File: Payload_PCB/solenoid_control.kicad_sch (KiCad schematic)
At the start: 9 parts, among them Q2 NMOS, Q29 NMOS

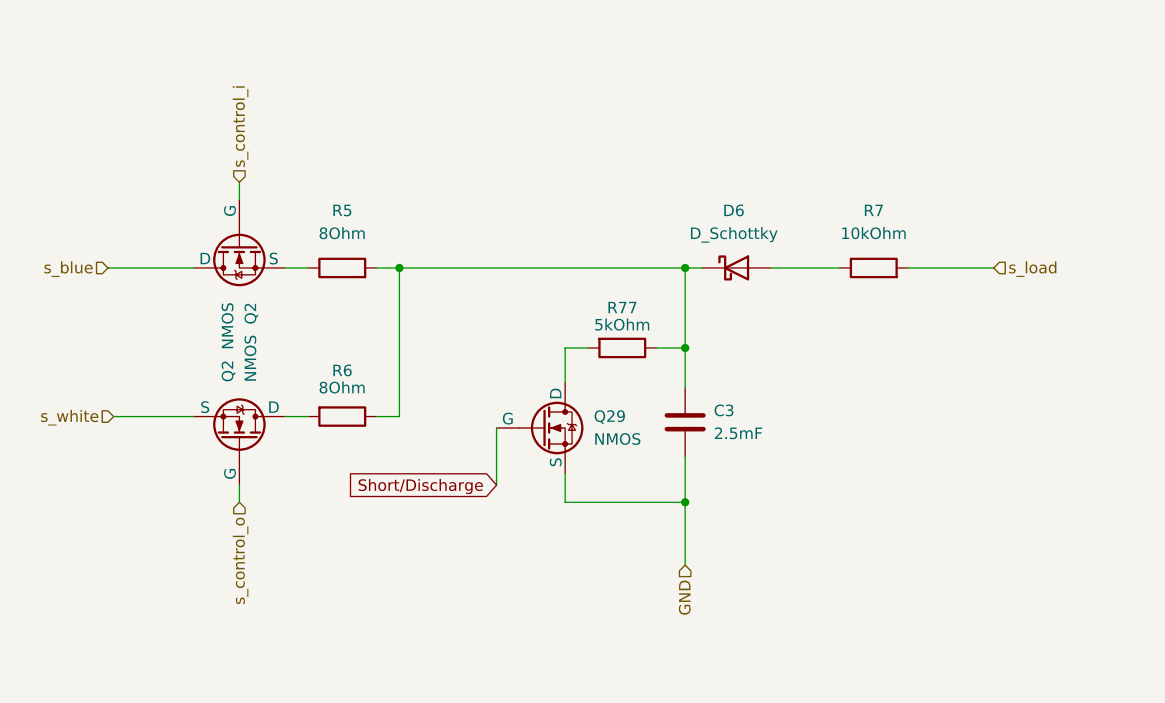
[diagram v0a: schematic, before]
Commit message: Added some actual parts
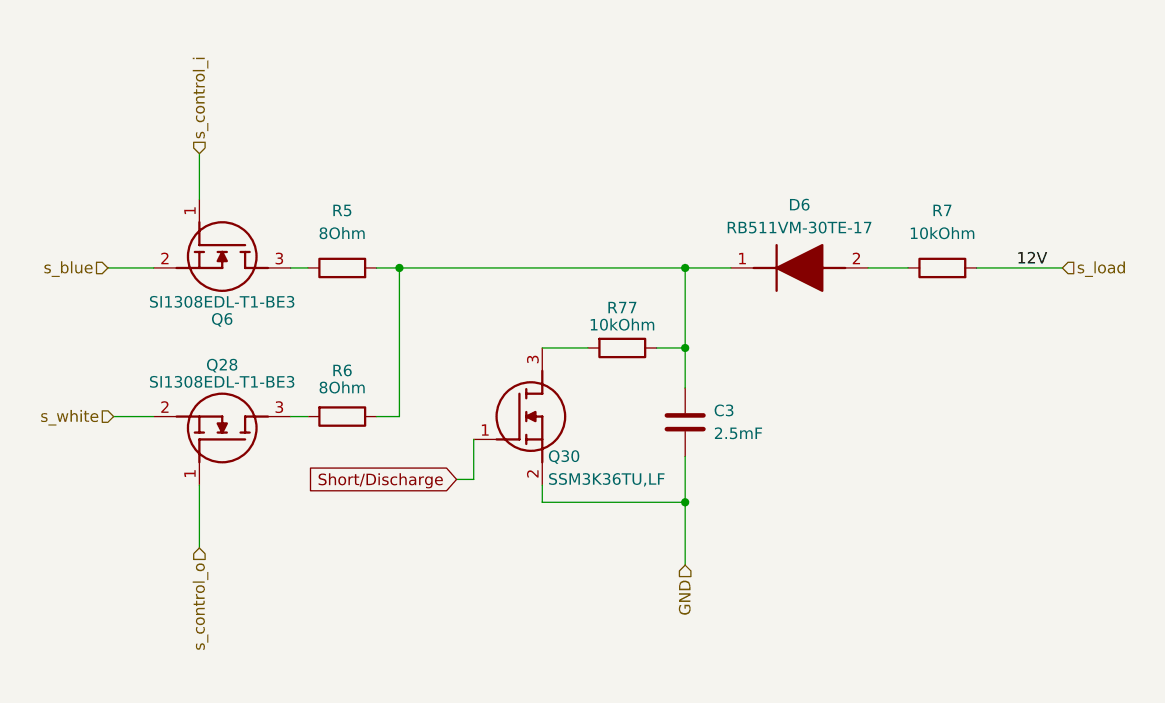
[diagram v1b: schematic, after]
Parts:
- removed D6: D_Schottky, symbol Device:D_Schottky
- removed Q2 (x2), Q29: NMOS, symbol Simulation_SPICE:NMOS
- added D6: RB511VM-30TE-17, RB511VM30TE17, symbol RB511VM-30TE-17:RB511VM-30TE-17
- added Q28, Q6: SI1308EDL-T1-BE3, SOT65P210X110-3N, symbol SI1308EDL-T1-BE3:SI1308EDL-T1-BE3
- added Q30: SSM3K36TU,LF, SOTFL65P210X75-3N, symbol SSM3K36TU_LF:SSM3K36TU,LF
- R77: value 5kOhm -> 10kOhm
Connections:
- net GND: now also Q30.2 (S)
- net Short/Discharge: now also Q30.1 (G)
- net s_blue: now also Q6.2 (S)
- net s_control_i: now also Q6.1 (G)
- net s_control_o: now also Q28.1 (G)
- net s_white: now also Q28.2 (S)
- net at R77.2: now also Q30.3 (D)
- net at R5.1: now also Q6.3 (D)
- net at C3.2, R5.2, R6.1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: now also D6.1 (K)
- net at R6.2: now also Q28.3 (D)
- net at R7.1: now also D6.2 (A)
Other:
- company: (none) -> SpaceTeam Aachen
- title: (none) -> Solenoid Control
- moved on the sheet: R7

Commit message: some new parts
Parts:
- D6: footprint RB511VM30TE17 -> footprints:RB511VM30TE17
- Q28, Q6: footprint SOT65P210X110-3N -> footprints:SOT65P210X110-3N
- Q30: footprint SOTFL65P210X75-3N -> footprints:SOTFL65P210X75-3N
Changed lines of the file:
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@@
       (effects (font (size 1.27 1.27)))
     )
-    (property "Footprint" "SOT65P210X110-3N" (at -32.69 66.675 0)
+    (property "Footprint" "footprints:SOT65P210X110-3N" (at -32.69 66.675 0)
       (effects (font (size 1.27 1.27)) (justify left top) hide)
     )
@@
       (effects (font (size 1.27 1.27)))
     )
-    (property "Footprint" "SOT65P210X110-3N" (at -32.69 57.785 0)
+    (property "Footprint" "footprints:SOT65P210X110-3N" (at -32.69 57.785 0)
       (effects (font (size 1.27 1.27)) (justify left top) hide)
     )
@@
       (effects (font (size 1.27 1.27)) (justify left))
     )
-    (property "Footprint" "SOTFL65P210X75-3N" (at 107.95 171.755 0)
+    (property "Footprint" "footprints:SOTFL65P210X75-3N" (at 107.95 171.755 0)
       (effects (font (size 1.27 1.27)) (justify left top) hide)
     )
@@
       (effects (font (size 1.27 1.27)))
     )
-    (property "Footprint" "RB511VM30TE17" (at 136.525 151.435 0)
-      (effects (font (size 1.27 1.27)) (justify left top) hide)
-    )
+    (property "Footprint" "footprints:RB511VM30TE17" (at 136.525 151.435 0)
+      (effects (font (size 1.27 1.27)) (justify left top) hide)
+    )
